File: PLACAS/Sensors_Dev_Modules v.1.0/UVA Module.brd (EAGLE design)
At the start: 25 x 25 mm, 5 parts

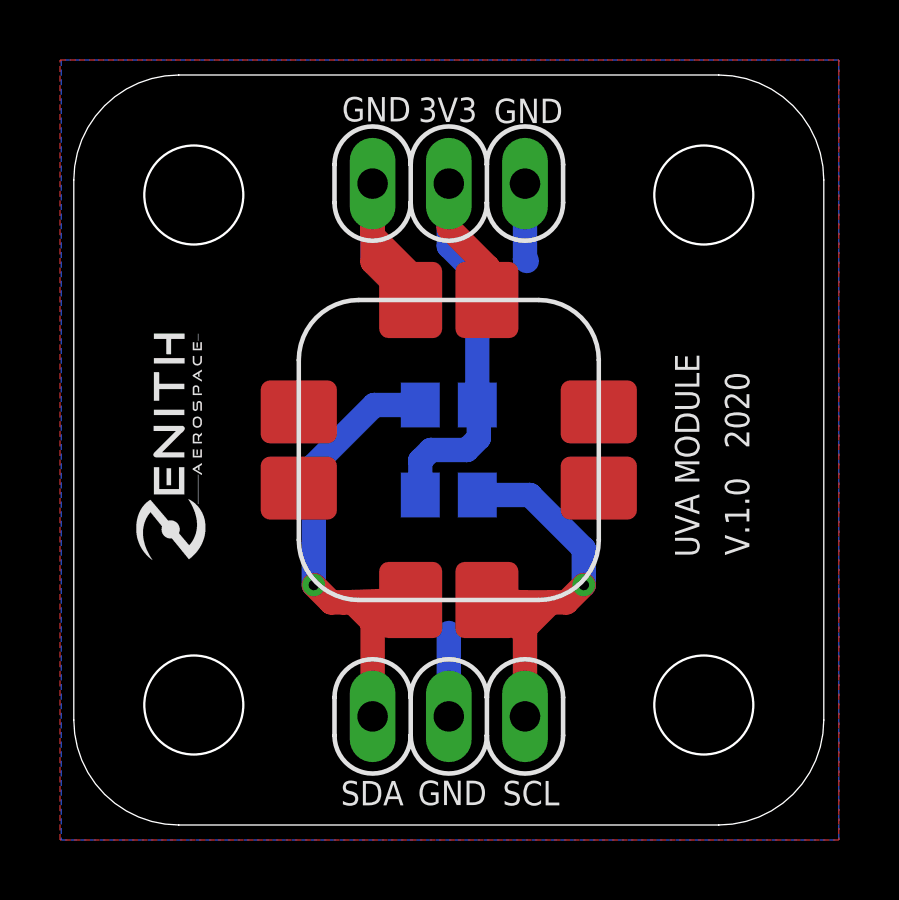
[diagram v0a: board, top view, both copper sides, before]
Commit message: Add files via upload
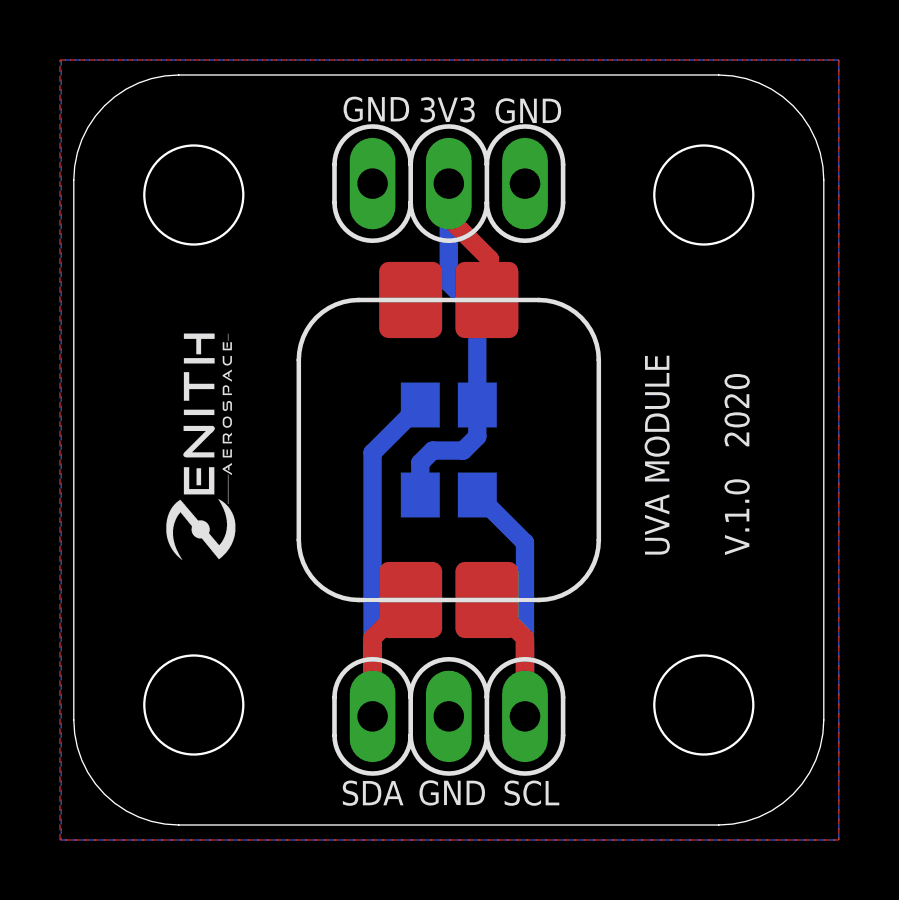
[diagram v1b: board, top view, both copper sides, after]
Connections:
- net GND: now also U$1.GND; no longer U$1.GND0, U$1.GND1, U$1.GND2, U$1.GND3, U$1.GND4
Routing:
- net GND: track 16.1 -> 0.00 mm
- net N$4: track 15.9 -> 17.9 mm, vias 1 -> 0
- net N$5: vias 1 -> 0
